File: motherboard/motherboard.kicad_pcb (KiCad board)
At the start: 2 copper layers, 32 x 55 mm, 21 parts, among them J1 532610471, J2 GSB1C41110SSHR, J3 532610471, J4 532610471, J5 532610471, J6 Conn_01x04_Pin, U1 RP2040, U2 ESP32-C3-WROOM-02U, U3 USBLC6-2SC6, U4 AP2112K-3.3TRG1

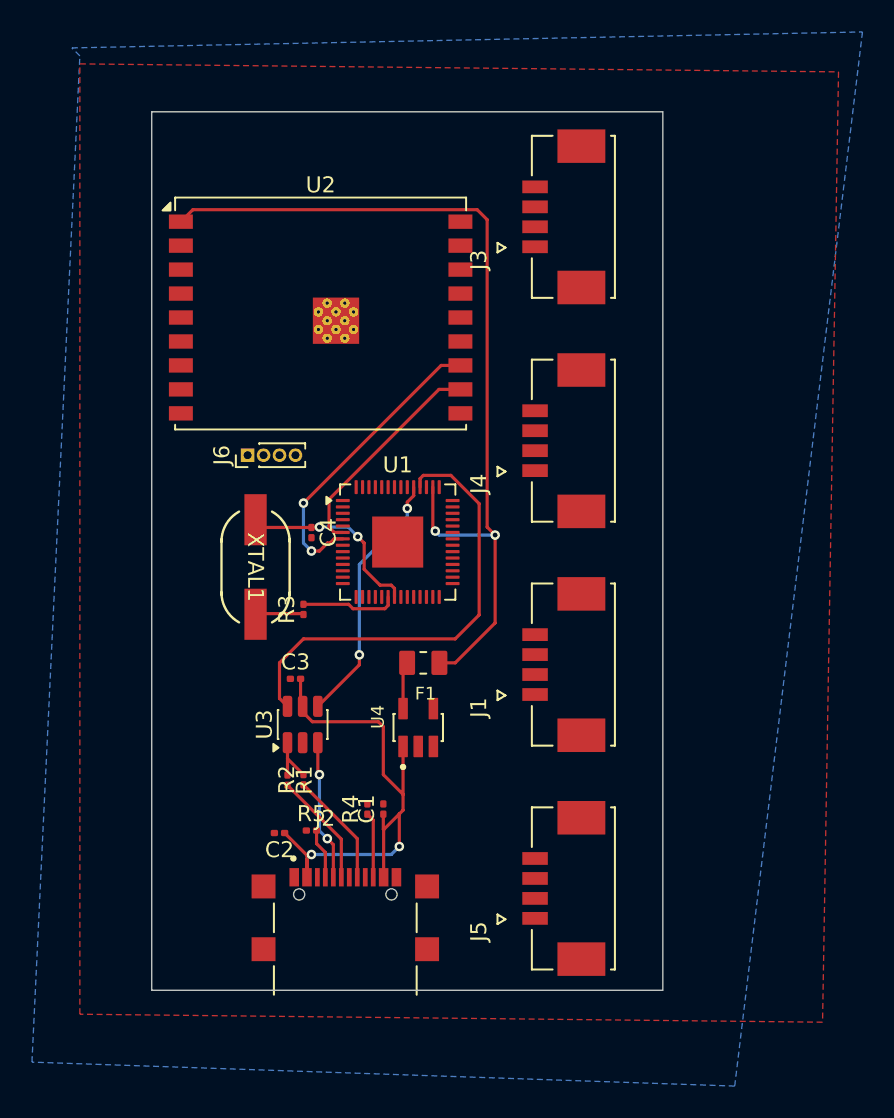
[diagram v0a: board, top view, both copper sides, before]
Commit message: fix : 3d model and footprint
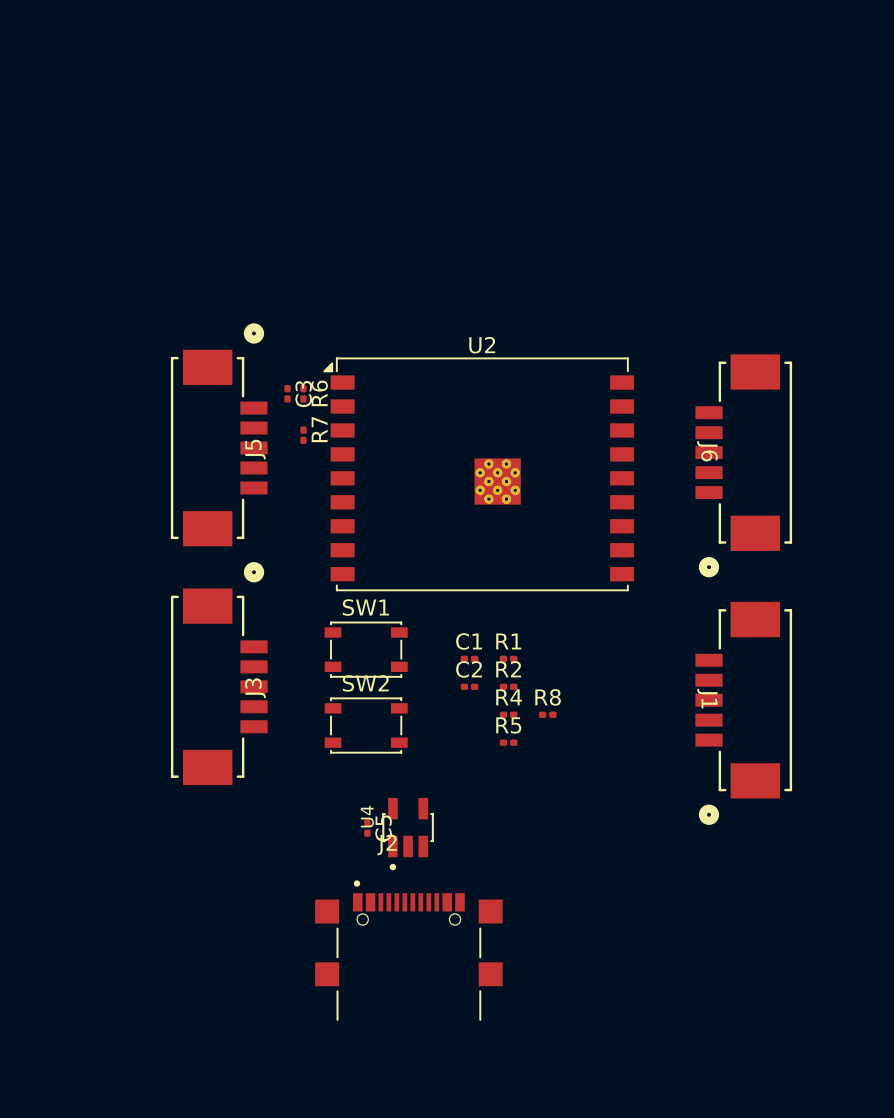
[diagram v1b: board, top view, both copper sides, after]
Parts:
- removed C4: 27pF, Capacitor_SMD:C_0201_0603Metric
- removed F1: 0ZCK0050FF2E, Library:FUSC2113X125N
- removed J4: 532610471, Library:MOLEX_532610471
- removed R3: 1kΩ, Resistor_SMD:R_0201_0603Metric
- removed U1: RP2040, Package_DFN_QFN:QFN-56-1EP_7x7mm_P0.4mm_EP3.2x3.2mm
- removed U3: USBLC6-2SC6, Package_TO_SOT_SMD:SOT-23-6
- removed XTAL1: ABLS7M2-12.000MHZ-D-2Y-T, footprints:XTAL_ABLS7M2_ABR
- added C5: 0.1µF, Capacitor_SMD:C_0201_0603Metric, F.Cu at (136.0, 130.8)
- added R6: 10 kΩ, Resistor_SMD:R_0201_0603Metric, F.Cu at (132.0, 103.7)
- added R7: 4.7 kΩ, Resistor_SMD:R_0201_0603Metric, F.Cu at (132.0, 106.2)
- added R8: 4.7 kΩ, Resistor_SMD:R_0201_0603Metric, F.Cu at (147.3, 123.8)
- added SW1: SW_Push, Button_Switch_SMD:SW_SPST_PTS810, F.Cu at (135.9, 119.7)
- added SW2: SW_Push, Button_Switch_SMD:SW_SPST_PTS810, F.Cu at (135.9, 124.4)
- C3: value 100nF -> 1µF
- J1, J3, J5: value 532610471 -> 532610571; footprint Library:MOLEX_532610471 -> footprint:CONN_532610001-SD_05_MOL
- J2: footprint Library:AMPHENOL_GSB1C41110SSHR -> footprint:AMPHENOL_GSB1C41110SSHR
- J6: value Conn_01x04_Pin -> 532610571; footprint Connector_PinHeader_1.00mm:PinHeader_1x04_P1.00mm_Vertical -> footprint:CONN_532610001-SD_05_MOL
- U4: footprint Library:SOT95P285X140-5N -> footprint:SOT95P285X140-5N
- moved J3 37.3 mm to (126.0, 122.0)
- moved J5 35.8 mm to (126.0, 107.0)
- moved J6 31.8 mm to (160.3, 107.3), turned to -90 degrees
- moved C3 17.9 mm to (131.0, 103.7), turned to -90 degrees
- moved R1 15.8 mm to (144.8, 120.2), turned to 0 degrees
- moved C2 15.0 mm to (142.4, 122.0), turned to 0 degrees
- moved U2 14.3 mm to (143.2, 109.0)
- moved R2 14.1 mm to (144.8, 122.0), turned to 0 degrees
- moved R5 13.5 mm to (144.8, 125.5)
- moved J1 11.6 mm to (160.3, 122.8), turned to -90 degrees
- moved C1 10.8 mm to (142.4, 120.2), turned to 0 degrees
- moved R4 10.6 mm to (144.8, 123.8), turned to 0 degrees
- moved U4 6.30 mm to (138.6, 130.8)
- moved J2 4.28 mm to (138.6, 139.2)
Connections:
- C1 pad 1: Net-(J2-VBUS_A) -> CLICK_2
- C2 pad 1: Net-(J2-VBUS_A) -> CLICK_2
- C3 pad 2: Net-(J2-VBUS_A) -> Net-(U2-EN)
- J1 pad 1: unconnected-(J1-Pad1) -> CLICK_1
- J1 pad 2: unconnected-(J1-Pad2) -> ADC_Y_1
- J1 pad 3: unconnected-(J1-Pad3) -> ADC_X_1
- J1 pad 4: unconnected-(J1-Pad4) -> CLICK_2
- J3 pad 2: unconnected-(J3-Pad2) -> SDA
- J3 pad 3: unconnected-(J3-Pad3) -> SCL
- J3 pad 4: unconnected-(J3-Pad4) -> CLICK_2
- J5 pad 2: unconnected-(J5-Pad2) -> SDA
- J5 pad 3: unconnected-(J5-Pad3) -> SCL
- J5 pad 4: unconnected-(J5-Pad4) -> CLICK_2
- J6 pad 1: unconnected-(J6-Pin_1-Pad1) -> CLICK_2
- J6 pad 2: unconnected-(J6-Pin_2-Pad2) -> ADC_Y_2
- J6 pad 3: unconnected-(J6-Pin_3-Pad3) -> ADC_X_2
- J6 pad 4: unconnected-(J6-Pin_4-Pad4) -> CLICK_2
- U2 pad 1: Net-(U1-VREG_IN) -> CLICK_2
- U2 pad 11: /TX -> unconnected-(U2-IO20/RXD-Pad11)
- U2 pad 12: /RX -> unconnected-(U2-IO21/TXD-Pad12)
- U2 pad 13: unconnected-(U2-IO18-Pad13) -> /D-
- U2 pad 14: unconnected-(U2-IO19-Pad14) -> /D+
- U2 pad 15: unconnected-(U2-IO3-Pad15) -> ADC_Y_2
- U2 pad 16: unconnected-(U2-IO2-Pad16) -> ADC_X_2
- U2 pad 17: unconnected-(U2-IO1-Pad17) -> ADC_Y_1
- U2 pad 18: unconnected-(U2-IO0-Pad18) -> ADC_X_1
- U2 pad 2: unconnected-(U2-EN-Pad2) -> Net-(U2-EN)
- U2 pad 3: unconnected-(U2-IO4-Pad3) -> CLICK_1
- U2 pad 4: unconnected-(U2-IO5-Pad4) -> CLICK_2
- U2 pad 7: unconnected-(U2-IO8-Pad7) -> SDA
- U2 pad 8: unconnected-(U2-IO9-Pad8) -> SCL
- U4 pad 3: unconnected-(U4-EN-Pad3) -> Net-(J2-VBUS_A)
- U4 pad 5: Net-(U4-VOUT) -> CLICK_2
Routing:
- net Net-(U1-VREG_IN): track 56.4 -> 0.00 mm, vias 2 -> 0
- net Net-(J2-VBUS_A): track 34.6 -> 0.00 mm, vias 2 -> 0
- net Net-(U1-USB_DM): track 28.7 -> 0.00 mm
- net /RX: track 18.9 -> 0.00 mm, vias 2 -> 0
- net Net-(U1-USB_DP): track 16.2 -> 0.00 mm, vias 2 -> 0
- net /TX: track 13.8 -> 0.00 mm
- net Net-(U1-XOUT): track 12.5 -> 0.00 mm, vias 2 -> 0
- net /D-: track 8.83 -> 0.00 mm, vias 2 -> 0
- net Net-(J2-DP2): track 7.18 -> 0.00 mm
- net Net-(J2-DP1): track 7.16 -> 0.00 mm
- net Net-(U1-XIN): track 6.03 -> 0.00 mm
- net Net-(J2-CC2): track 4.10 -> 0.00 mm
- net Net-(R3-Pad1): track 3.52 -> 0.00 mm
- net /D+: track 3.44 -> 0.00 mm
- net Net-(J2-CC1): track 3.15 -> 0.00 mm
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- removed copper zone on B.Cu, net GND
- removed copper zone on F.Cu, net GND
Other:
- board outline removed
